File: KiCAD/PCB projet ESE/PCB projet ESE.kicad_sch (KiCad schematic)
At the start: 49 parts, among them J1 Conn_01x06, J2 Conn_01x04, J3 Conn_01x06, J4 Conn_01x06, J5 Conn_01x02, J6 Conn_01x04, J7 Conn_ST_STDC14, SW1 SW_SPST, SW2 472121010111, U1 ZXBM5210-SP, U2 ZXBM5210-SP, U3 STM32G474RETx, U4 ADXL343

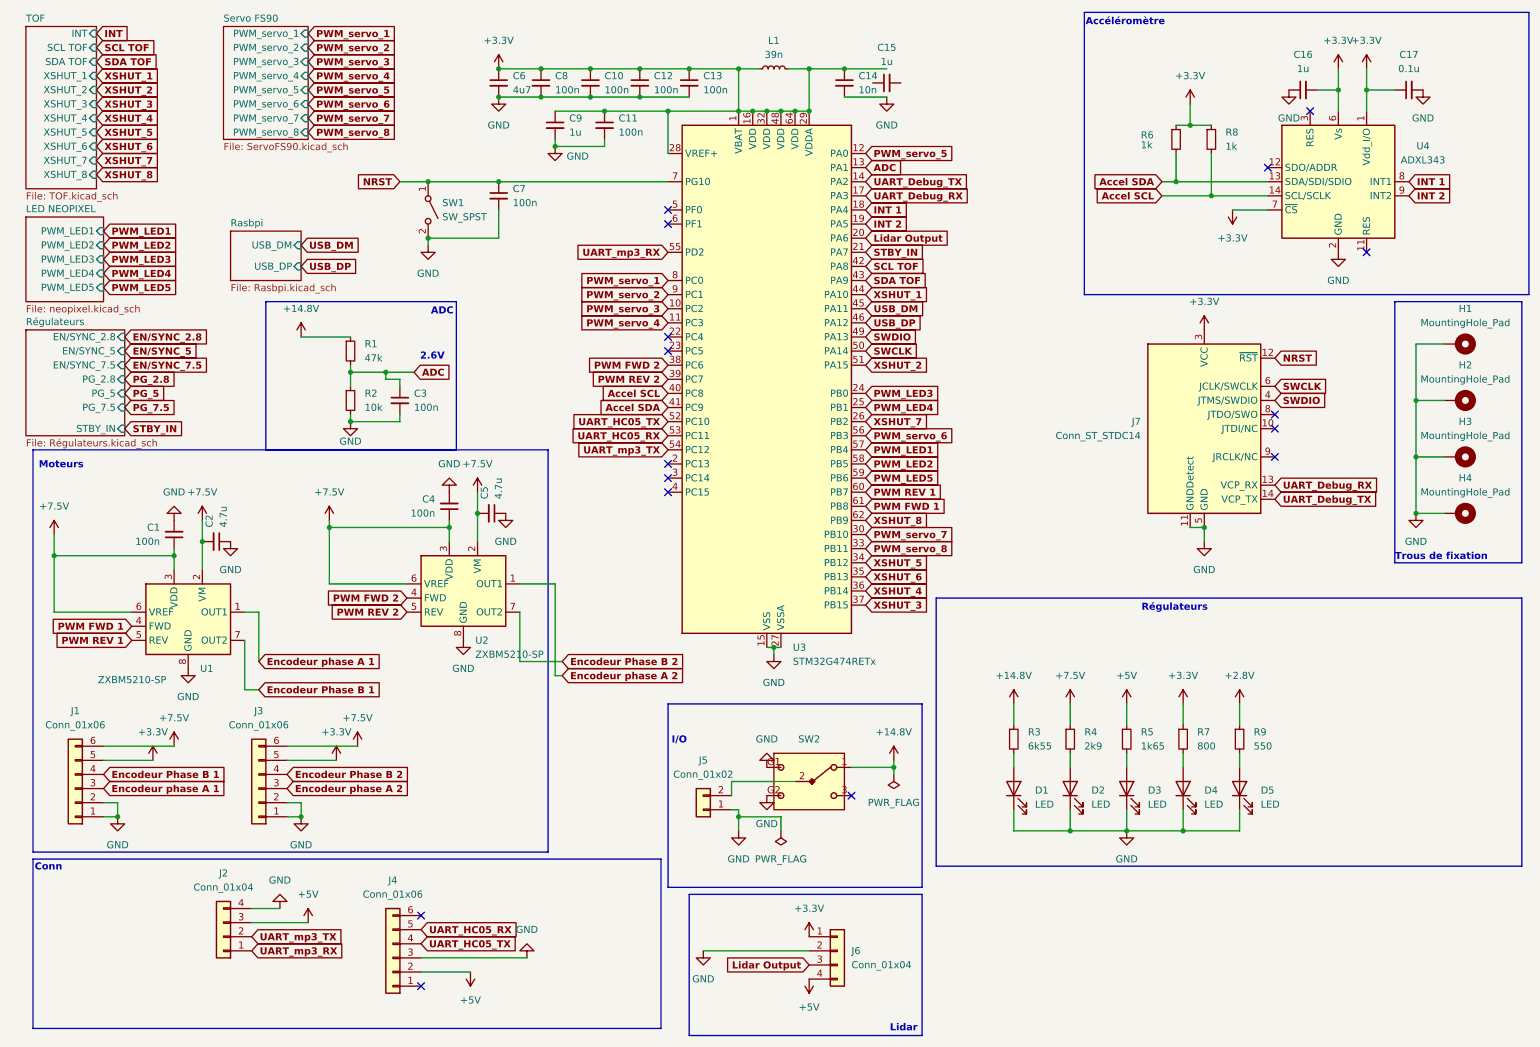
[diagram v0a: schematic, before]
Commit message: maj scgematic
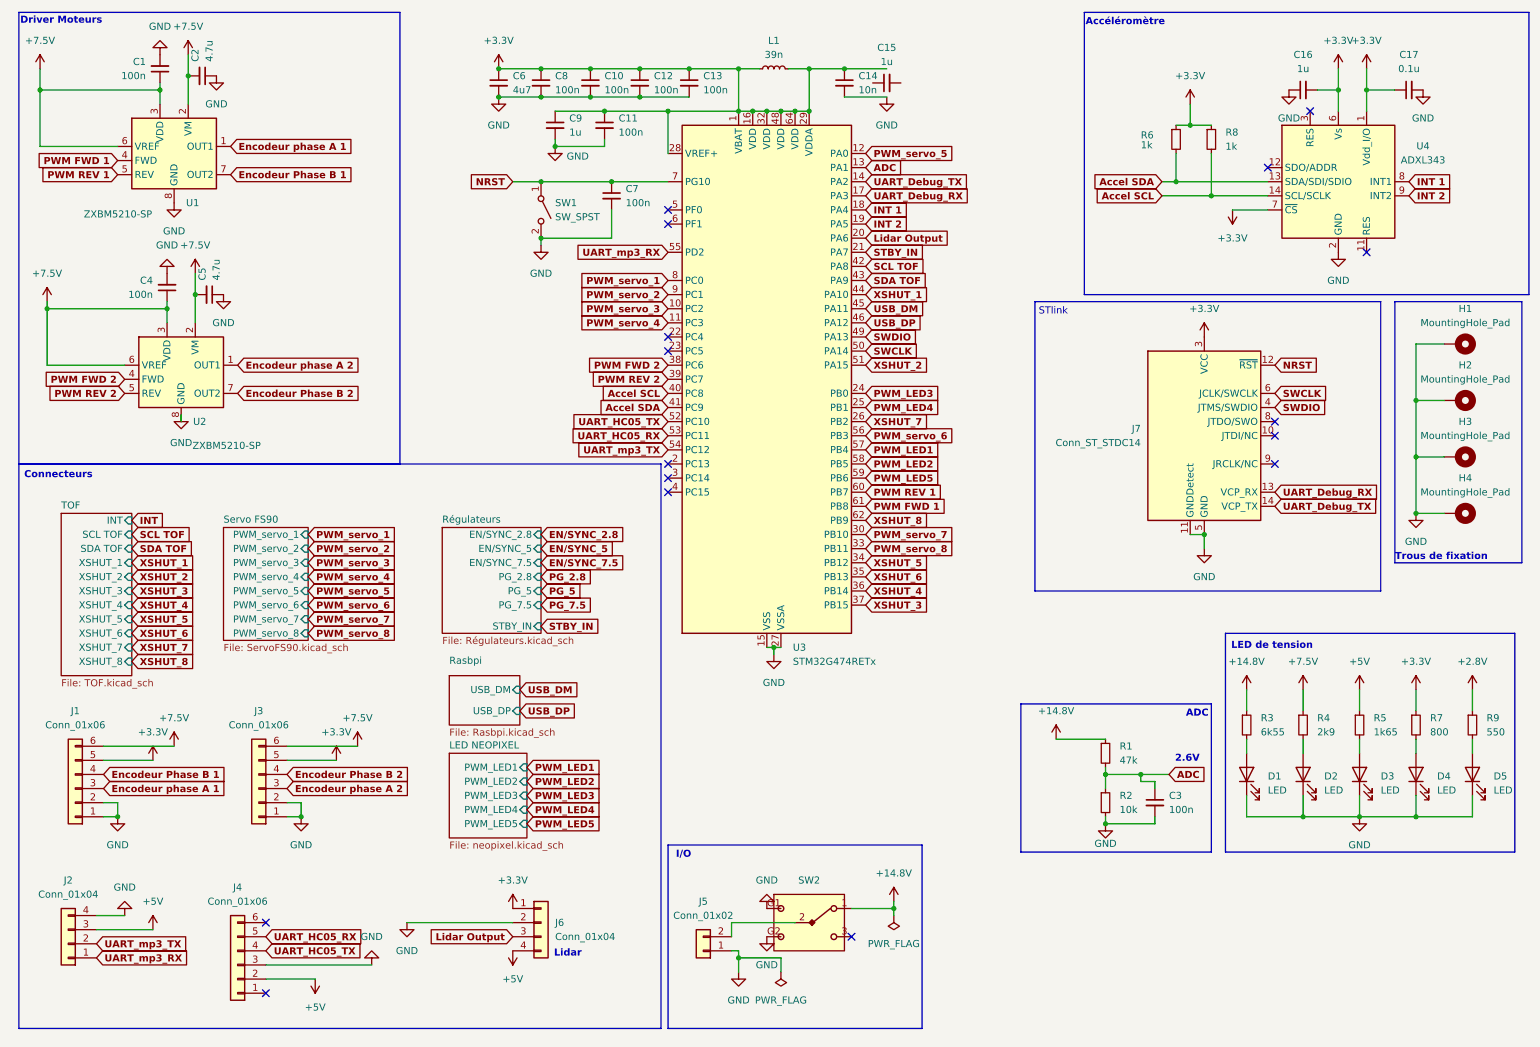
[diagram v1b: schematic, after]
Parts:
- SW2: MPN (none) -> 472123020421
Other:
- note added: "Connecteurs"
- note added: "Driver Moteurs"
- note added: "LED de tension"
- note added: "STlink"
- note removed: "Conn"
- note removed: "Moteurs"
- note removed: "Régulateurs"
- moved on the sheet: C1, C2, C3, C4, C5, C7, D1, D2, D3, D4, D5, J2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
